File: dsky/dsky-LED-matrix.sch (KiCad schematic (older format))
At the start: 53 parts, among them U26 IS31FL3236A

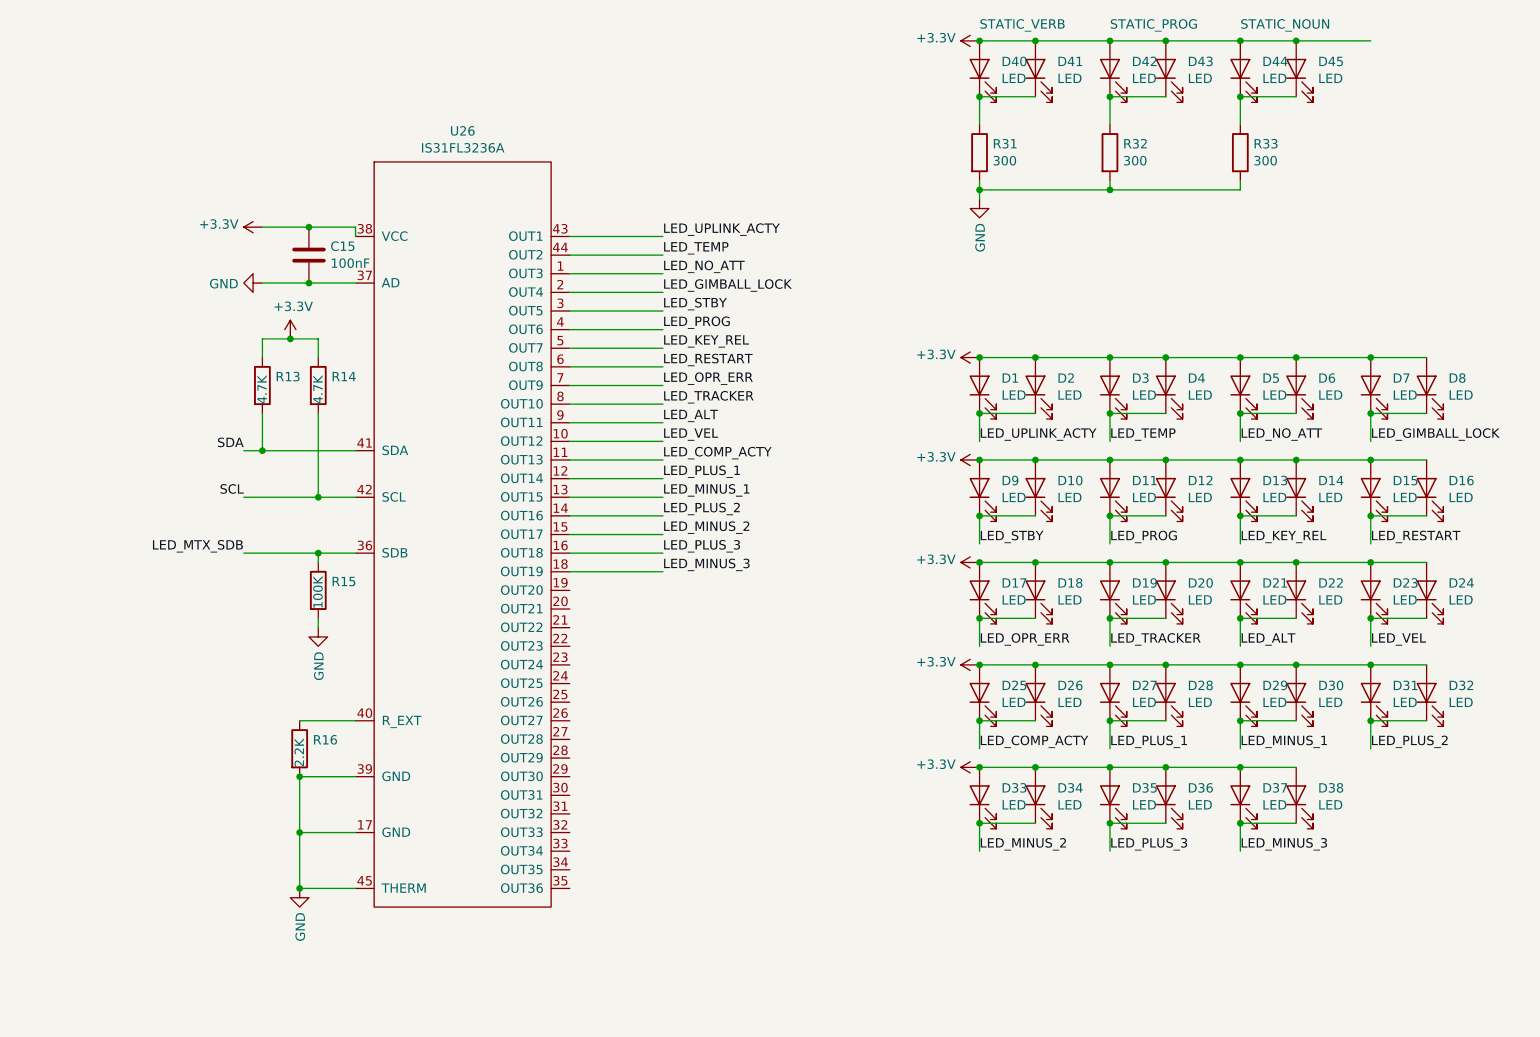
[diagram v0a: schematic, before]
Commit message: this hard drive is dying
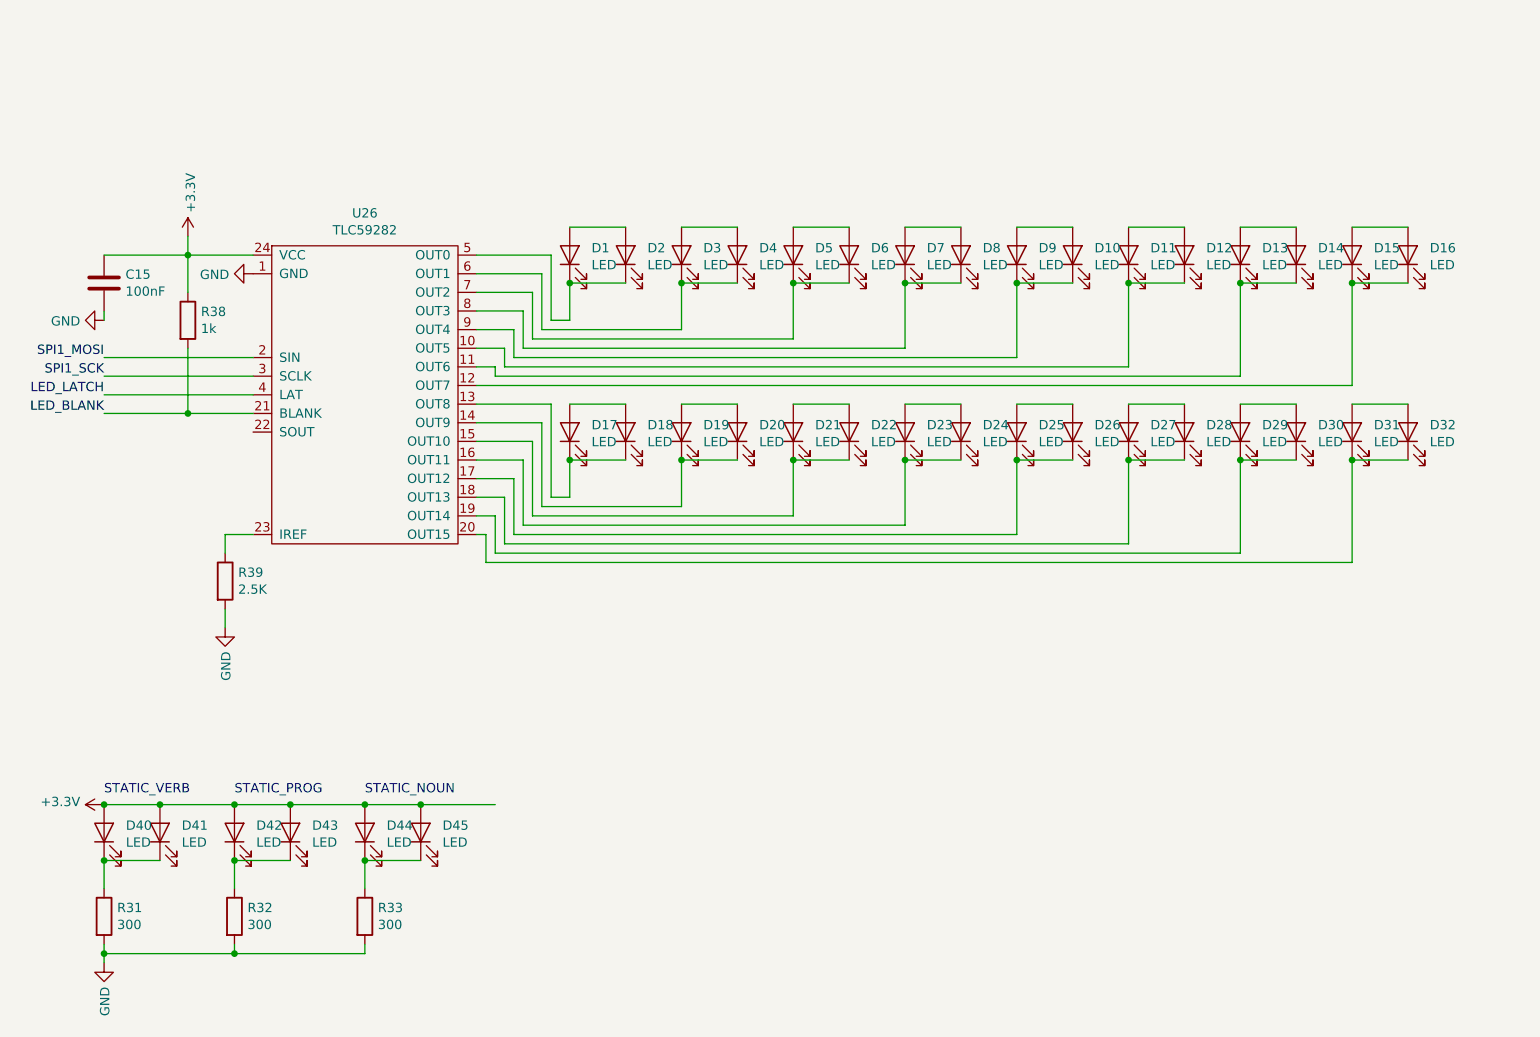
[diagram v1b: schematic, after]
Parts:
- removed D33, D34, D35, D36, D37, D38: LED, dsky:2.00x0.50_RIGHT_LED, symbol Device:LED
- removed R13, R14: 4.7K, Resistor_SMD:R_0603_1608Metric, symbol Device:R
- removed R15: 100K, Resistor_SMD:R_0603_1608Metric, symbol Device:R
- removed R16: 2.2K, Resistor_SMD:R_0603_1608Metric, symbol Device:R
- removed U26: IS31FL3236A, symbol dsky:IS31FL3236A
- added R38: 1k, Resistor_SMD:R_0402_1005Metric, symbol Device:R
- added R39: 2.5K, Resistor_SMD:R_0402_1005Metric, symbol Device:R
- added U26: TLC59282, Package_SO:SSOP-24_3.9x8.7mm_P0.635mm, symbol dsky:TLC59282
- C15: footprint Capacitor_SMD:C_0603_1608Metric -> Capacitor_SMD:C_0402_1005Metric
- R31, R32, R33: footprint Resistor_SMD:R_0805_2012Metric -> Resistor_SMD:R_0603_1608Metric
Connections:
- net +3V3: now also R38.1, U26.24 (VCC); no longer D1.2 (A), D10.2 (A), D11.2 (A), D12.2 (A), D13.2 (A), D14.2 (A), D15.2 (A), D16.2 (A), D17.2 (A), D18.2 (A), D19.2 (A), D2.2 (A), D20.2 (A), D21.2 (A), D22.2 (A), D23.2 (A), D24.2 (A), D25.2 (A), D26.2 (A), D27.2 (A), D28.2 (A), D29.2 (A), D3.2 (A), D30.2 (A), D31.2 (A), D32.2 (A), D4.2 (A), D5.2 (A), D6.2 (A), D7.2 (A), D8.2 (A), D9.2 (A)
- net GND: now also R39.2, U26.1 (GND)
- net LED_ALT: no longer names the net of D21.1 (K), D22.1 (K)
- net LED_ALT: now also U26.15 (OUT10)
- net LED_COMP_ACTY: no longer names the net of D25.1 (K), D26.1 (K)
- net LED_COMP_ACTY: now also U26.17 (OUT12)
- net LED_GIMBALL_LOCK: no longer names the net of D7.1 (K), D8.1 (K)
- net LED_GIMBALL_LOCK: now also U26.8 (OUT3)
- net LED_KEY_REL: no longer names the net of D13.1 (K), D14.1 (K)
- net LED_KEY_REL: now also U26.11 (OUT6)
- net LED_MINUS_1: no longer names the net of D29.1 (K), D30.1 (K)
- net LED_MINUS_1: now also U26.19 (OUT14)
- net LED_NO_ATT: no longer names the net of D5.1 (K), D6.1 (K)
- net LED_NO_ATT: now also U26.7 (OUT2)
- net LED_OPR_ERR: no longer names the net of D17.1 (K), D18.1 (K)
- net LED_OPR_ERR: now also U26.13 (OUT8)
- net LED_PLUS_1: no longer names the net of D27.1 (K), D28.1 (K)
- net LED_PLUS_1: now also U26.18 (OUT13)
- net LED_PLUS_2: no longer names the net of D31.1 (K), D32.1 (K)
- net LED_PLUS_2: now also U26.20 (OUT15)
- net LED_PROG: no longer names the net of D11.1 (K), D12.1 (K)
- net LED_PROG: now also U26.10 (OUT5)
- net LED_RESTART: no longer names the net of D15.1 (K), D16.1 (K)
- net LED_RESTART: now also U26.12 (OUT7)
- net LED_STBY: no longer names the net of D10.1 (K), D9.1 (K)
- net LED_STBY: now also U26.9 (OUT4)
- net LED_TEMP: no longer names the net of D3.1 (K), D4.1 (K)
- net LED_TEMP: now also U26.6 (OUT1)
- net LED_TRACKER: no longer names the net of D19.1 (K), D20.1 (K)
- net LED_TRACKER: now also U26.14 (OUT9)
- net LED_UPLINK_ACTY: no longer names the net of D1.1 (K), D2.1 (K)
- net LED_UPLINK_ACTY: now also U26.5 (OUT0)
- net LED_VEL: no longer names the net of D23.1 (K), D24.1 (K)
- net LED_VEL: now also U26.16 (OUT11)
- new net: R39.1, U26.23 (IREF)
- new net: D1.2 (A), D2.2 (A)
- new net: D10.2 (A), D9.2 (A)
- new net: D3.2 (A), D4.2 (A)
- new net: D11.2 (A), D12.2 (A)
- new net: D5.2 (A), D6.2 (A)
- new net: D13.2 (A), D14.2 (A)
- new net: D7.2 (A), D8.2 (A)
- new net: D15.2 (A), D16.2 (A)
- new net: D17.2 (A), D18.2 (A)
- new net: D25.2 (A), D26.2 (A)
- new net: D19.2 (A), D20.2 (A)
- new net: D27.2 (A), D28.2 (A)
- new net: D21.2 (A), D22.2 (A)
- new net: D29.2 (A), D30.2 (A)
- new net: D23.2 (A), D24.2 (A)
- new net: D31.2 (A), D32.2 (A)
- new net LED_BLANK: R38.2, U26.21 (BLANK)
- new net LED_LATCH: U26.4 (LAT)
- new net SPI1_MOSI: U26.2 (SIN)
- new net SPI1_SCK: U26.3 (SCLK)
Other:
- moved on the sheet: C15, D1, D10, D11, D12, D13, D14, D15, D16, D17, D18, D19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
